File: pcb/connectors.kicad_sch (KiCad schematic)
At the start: 8 parts, among them J1 USB_C_Receptacle_USB2.0, U6 USBLC6-2SC6

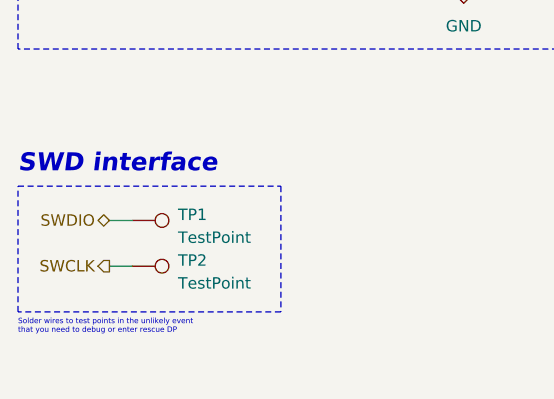
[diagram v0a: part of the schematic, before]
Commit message: PCB design complete
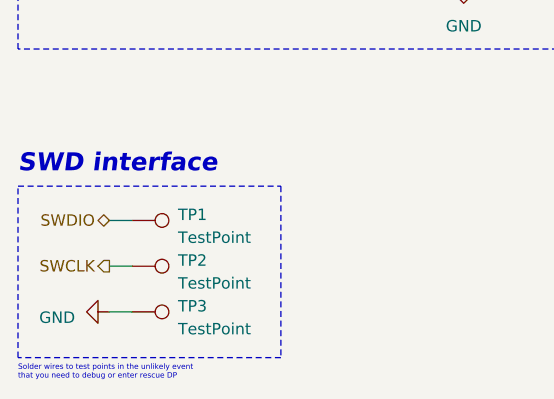
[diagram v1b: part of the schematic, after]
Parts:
- added TP3: TestPoint, TestPoint:TestPoint_Pad_D2.0mm, symbol Connector:TestPoint
- R8: LCSC (none) -> C25744
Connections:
- net GND: now also TP3.1
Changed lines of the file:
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@@
+    (stroke (width 0) (type default))
+  )
+  (wire (pts (xy 35.56 115.57) (xy 38.1 115.57))
     (stroke (width 0) (type default))
   )
@@
     (fill (type none))
   )
-  (rectangle (start 25.4 101.6) (end 54.61 115.57)
+  (rectangle (start 25.4 101.6) (end 54.61 120.65)
     (stroke (width 0) (type dash))
     (fill (type none))
   )
   (text "Solder wires to test points in the unlikely event\nthat you need to debug or enter rescue DP"
-    (at 25.4 118.11 0)
+    (at 25.4 123.19 0)
     (effects (font (size 0.6 0.6)) (justify left bottom))
   )
@@
   (hierarchical_label "USB_D-" (shape bidirectional) (at 80.01 40.64 0) (fields_autoplaced)
     (effects (font (size 1.27 1.27)) (justify left))
+  )
+  (symbol (lib_id "Connector:TestPoint") (at 38.1 115.57 270) (unit 1)
+    (in_bom yes) (on_board yes) (dnp no) (fields_autoplaced)
+    (property "Reference" "TP3" (at 43.18 114.935 90)
+      (effects (font (size 1.27 1.27)) (justify left))
+    )
+    (property "Value" "TestPoint" (at 43.18 117.475 90)
+      (effects (font (size 1.27 1.27)) (justify left))
+    )
+    (property "Footprint" "TestPoint:TestPoint_Pad_D2.0mm" (at 38.1 120.65 0)
+      (effects (font (size 1.27 1.27)) hide)
+    )
+    (property "Datasheet" "~" (at 38.1 120.65 0)
+      (effects (font (size 1.27 1.27)) hide)
+    )
+    (pin "1")
+    (instances
+      (project "keyboard"
+        (path "/fc529d87-72d0-4c92-b352-ddcf4c6f7199/953c467c-8c0d-4158-80e9-7f51ef1515ee"
+          (reference "TP3") (unit 1)
+        )
+      )
+    )
   )
   (symbol (lib_id "Power_Protection:USBLC6-2SC6") (at 76.2 50.8 270) (unit 1)
@@
       (effects (font (size 1.27 1.27)) hide)
     )
+    (property "LCSC" "C25744" (at 60.96 72.39 0)
+      (effects (font (size 1.27 1.27)) hide)
+    )
     (pin "1")
     (pin "2")
@@
       (effects (font (size 1.27 1.27)) hide)
     )
+    (property "LCSC" "C25744" (at 83.82 72.39 0)
+      (effects (font (size 1.27 1.27)) hide)
+    )
     (pin "1")
     (pin "2")
@@
         (path "/fc529d87-72d0-4c92-b352-ddcf4c6f7199/953c467c-8c0d-4158-80e9-7f51ef1515ee"
           (reference "R4") (unit 1)
+        )
+      )
+    )
+  )
+  (symbol (lib_id "power:GND") (at 35.56 115.57 270) (unit 1)
+    (in_bom yes) (on_board yes) (dnp no) (fields_autoplaced)
+    (property "Reference" "#PWR025" (at 29.21 115.57 0)
+      (effects (font (size 1.27 1.27)) hide)
+    )
+    (property "Value" "GND" (at 31.75 116.205 90)
+      (effects (font (size 1.27 1.27)) (justify right))
+    )
+    (property "Footprint" "" (at 35.56 115.57 0)
+      (effects (font (size 1.27 1.27)) hide)
+    )
+    (property "Datasheet" "" (at 35.56 115.57 0)
+      (effects (font (size 1.27 1.27)) hide)
+    )
+    (pin "1")
+    (instances
+      (project "keyboard"
+        (path "/fc529d87-72d0-4c92-b352-ddcf4c6f7199/953c467c-8c0d-4158-80e9-7f51ef1515ee"
+          (reference "#PWR025") (unit 1)
         )
       )
@@
       (effects (font (size 1.27 1.27)) hide)
     )
+    (property "LCSC" "C25744" (at 66.04 72.39 0)
+      (effects (font (size 1.27 1.27)) hide)
+    )
     (pin "1")
     (pin "2")
@@
       (effects (font (size 1.27 1.27)) hide)
     )
+    (property "LCSC" "C25744" (at 88.9 72.39 0)
+      (effects (font (size 1.27 1.27)) hide)
+    )
